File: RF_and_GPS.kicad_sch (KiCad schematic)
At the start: 44 parts, among them J22 U.FL-R-SMT-1, J23 U.FL-R-SMT-1, J24 Conn_02x05_Odd_Even, Q1 IRLML2803, Q18 IRLML2803, Q19 IRF7404, Q22 IRLML2803, Q23 IRF7404, SW2 KMR231NG LFS, U10 ATSAMD21E18A-A, U11 MAX706RESA+, U12 E22-900M30S, U13 S1216V8, U14 EP2W+, Y2 32.768kHz

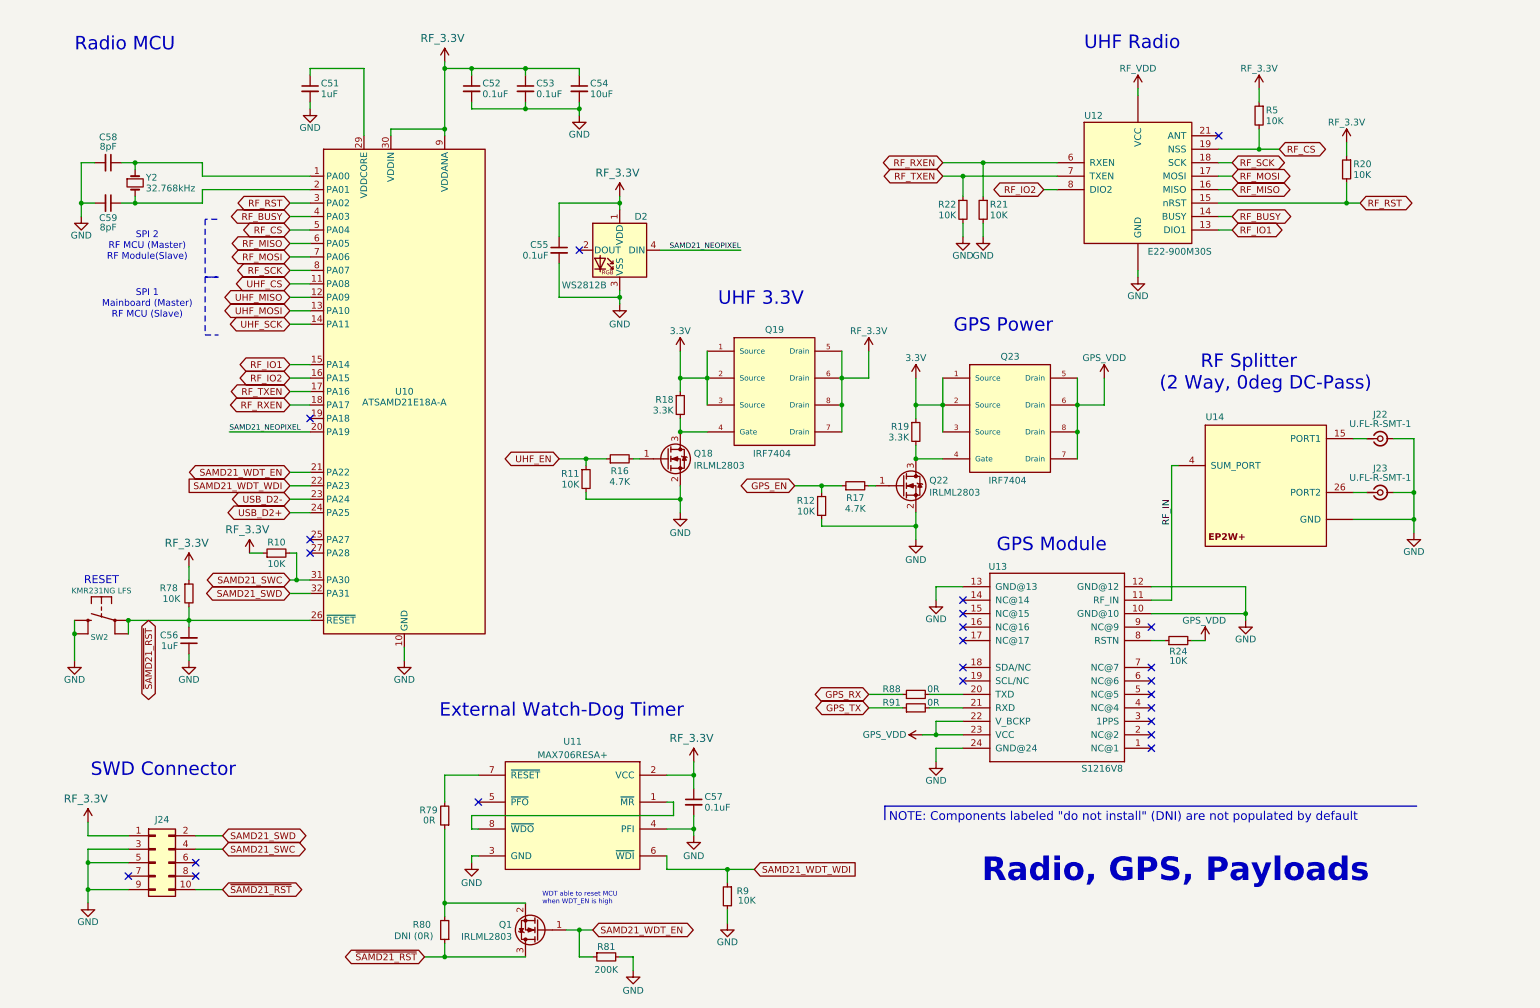
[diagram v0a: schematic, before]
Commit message: v1.1 Schematic
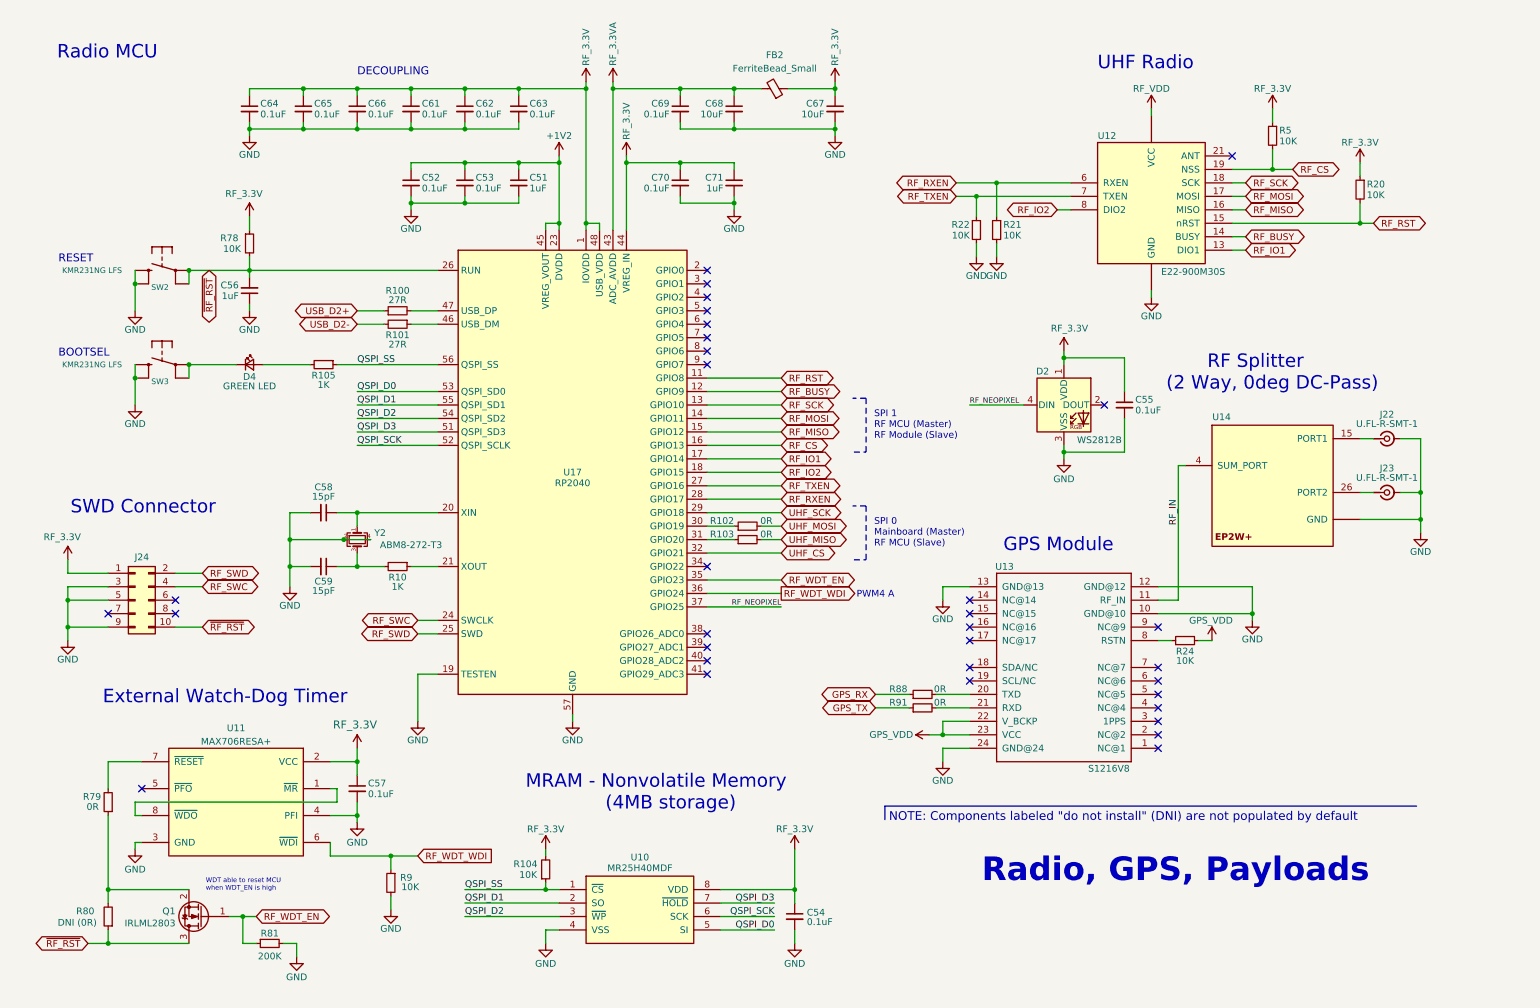
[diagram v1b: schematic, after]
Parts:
- removed Q18, Q22: IRLML2803, Package_TO_SOT_SMD:SOT-23, symbol Mainboard:IRLML2803
- removed Q19, Q23: IRF7404, Package_SO:SOIC-8_3.9x4.9mm_P1.27mm, symbol Mainboard:IRF7404
- removed R11, R12: 10K, Resistor_SMD:R_0603_1608Metric, symbol Device:R_Small
- removed R16, R17: 4.7K, Resistor_SMD:R_0603_1608Metric, symbol Device:R_Small
- removed R18, R19: 3.3K, Resistor_SMD:R_0603_1608Metric, symbol Device:R_Small
- removed U10: ATSAMD21E18A-A, Package_QFP:TQFP-32_7x7mm_P0.8mm, symbol MCU_Microchip_SAMD:ATSAMD21E18A-A
- removed Y2: 32.768kHz, Crystal:Crystal_SMD_3215-2Pin_3.2x1.5mm, symbol Device:Crystal_Small
- added C61, C62, C63, C64, C65, C66, C69, C70: 0.1uF, Capacitor_SMD:C_0603_1608Metric, symbol Device:C_Small
- added C67, C68: 10uF, Capacitor_SMD:C_0603_1608Metric, symbol Device:C_Small
- added C71: 1uF, Capacitor_SMD:C_0603_1608Metric, symbol Device:C_Small
- added D4: GREEN LED, LED_SMD:LED_0603_1608Metric, symbol Device:LED_Small
- added FB2: FerriteBead_Small, Inductor_SMD:L_0603_1608Metric, symbol Device:FerriteBead_Small
- added R100, R101: 27R, Resistor_SMD:R_0603_1608Metric, symbol Device:R_Small
- added R102, R103: 0R, Resistor_SMD:R_0603_1608Metric, symbol Device:R_Small
- added R104: 10K, Resistor_SMD:R_0603_1608Metric, symbol Device:R_Small
- added R105: 1K, Resistor_SMD:R_0603_1608Metric, symbol Device:R_Small
- added SW3: KMR231NG LFS, Button_Switch_SMD:SW_Push_1P1T_NO_CK_KMR2, symbol Mainboard:KMR231
- added U10: MR25H40MDF, Package_DFN_QFN:DFN-8-1EP_6x5mm_P1.27mm_EP2x2mm, symbol Mainboard:MR25H40MDF
- added U17: RP2040, Package_DFN_QFN:QFN-56-1EP_7x7mm_P0.4mm_EP3.2x3.2mm, symbol MCU_RaspberryPi:RP2040
- added Y2: ABM8-272-T3, Crystal:Crystal_SMD_3225-4Pin_3.2x2.5mm, symbol Device:Crystal_GND24_Small
- C54: value 10uF -> 0.1uF
- C58, C59: value 8pF -> 15pF
- R10: value 10K -> 1K
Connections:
- net GND: now also C61.2, C62.2, C63.2, C64.2, C65.2, C66.2, C67.2, C68.2, C69.2, C70.2, C71.2, SW3.2 (S1), U10.4 (VSS), U10.9 (EP), U17.19 (TESTEN), U17.57 (GND), Y2.2, Y2.4
- net RF_3.3V: now also C61.1, C62.1, C63.1, C64.1, C65.1, C66.1, C67.1, C70.1, C71.1, FB2.1, R104.2, U10.8 (VDD), U17.1 (IOVDD), U17.10 (IOVDD), U17.22 (IOVDD), U17.33 (IOVDD), U17.42 (IOVDD), U17.44 (VREG_IN), U17.48 (USB_VDD), U17.49 (IOVDD); no longer C52.1, C53.1, R10.1
- net RF_BUSY: now also U17.12 (GPIO9)
- net RF_CS: now also U17.16 (GPIO13)
- net RF_IO1: now also U17.17 (GPIO14)
- net RF_IO2: now also U17.18 (GPIO15)
- net RF_MISO: now also U17.15 (GPIO12)
- net RF_MOSI: now also U17.14 (GPIO11)
- net RF_RST: now also U17.11 (GPIO8)
- net RF_RXEN: now also U17.28 (GPIO17)
- net RF_SCK: now also U17.13 (GPIO10)
- net RF_TXEN: now also U17.27 (GPIO16)
- net UHF_CS: now also U17.32 (GPIO21)
- net UHF_MISO: now also R103.2
- net UHF_MOSI: now also R102.2
- net UHF_SCK: now also U17.29 (GPIO18)
- net USB_D2+: now also R100.1
- net USB_D2-: now also R101.2
- net at C58.1: now also U17.20 (XIN), Y2.1
- net at C59.1: now also R10.2, Y2.3
- net +1V2: now reaches C51.1
- net +1V2: now also C52.1, C53.1, U17.23 (DVDD), U17.45 (VREG_VOUT), U17.50 (DVDD)
- net SAMD21_NEOPIXEL renamed RF_NEOPIXEL
- net RF_NEOPIXEL: now also U17.37 (GPIO25)
- net SAMD21_SWC renamed RF_SWC
- net RF_SWC: now also U17.24 (SWCLK); no longer R10.2
- net SAMD21_SWD renamed RF_SWD
- net RF_SWD: now also U17.25 (SWD)
- net SAMD21_WDT_EN renamed RF_WDT_EN
- net RF_WDT_EN: now also U17.35 (GPIO23)
- net SAMD21_WDT_WDI renamed RF_WDT_WDI
- net RF_WDT_WDI: now also U17.36 (GPIO24)
- net ~{SAMD21_RST} renamed ~{RF_RST}
- net ~{RF_RST}: now also U17.26 (RUN)
- new net: R10.1, U17.21 (XOUT)
- new net: D4.1 (K), SW3.1 (P1)
- new net: R102.1, U17.30 (GPIO19)
- new net: R101.1, U17.46 (USB_DM)
- new net: D4.2 (A), R105.2
- new net: R100.2, U17.47 (USB_DP)
- new net: R103.1, U17.31 (GPIO20)
- new net QSPI_D0: U10.5 (SI), U17.53 (QSPI_SD0)
- new net QSPI_D1: U10.2 (SO), U17.55 (QSPI_SD1)
- new net QSPI_D2: U10.3 (~{WP}), U17.54 (QSPI_SD2)
- new net QSPI_D3: U10.7 (~{HOLD}), U17.51 (QSPI_SD3)
- new net QSPI_SCK: U10.6 (SCK), U17.52 (QSPI_SCLK)
- new net QSPI_SS: R104.1, R105.1, U10.1 (~{CS}), U17.56 (QSPI_SS)
- new net RF_3.3VA: C68.1, C69.1, FB2.2, U17.43 (ADC_AVDD)
- no-connect marks 23 -> 33
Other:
- note added: "BOOTSEL"
- note added: "DECOUPLING"
- note added: "MRAM - Nonvolatile Memory (4MB storage)"
- note added: "PWM4 A"
- note added: "SPI 0 Mainboard (Master) RF MCU (Slave)"
- note added: "SPI 1 RF MCU (Master) RF Module (Slave)"
- note removed: "GPS Power"
- note removed: "SPI 1 Mainboard (Master) RF MCU (Slave)"
- note removed: "SPI 2 RF MCU (Master) RF Module(Slave)"
- note removed: "UHF 3.3V"
- moved on the sheet: C51, C52, C53, C55, C56, C57, C58, C59, D2, J22, J23, J24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
